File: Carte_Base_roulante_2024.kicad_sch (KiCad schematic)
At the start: 33 parts, among them J1 Screw_Terminal_01x02, J16 Screw_Terminal_01x02, J2 Screw_Terminal_01x02, J26 Conn_01x04_Male, J27 Conn_01x04_Male, J28 Conn_01x04_Male, J3 Screw_Terminal_01x02, J8 USB_B_Micro, J9 Conn_01x05, U1 STM32G484RETx, U4 R-78E5.0-1.0

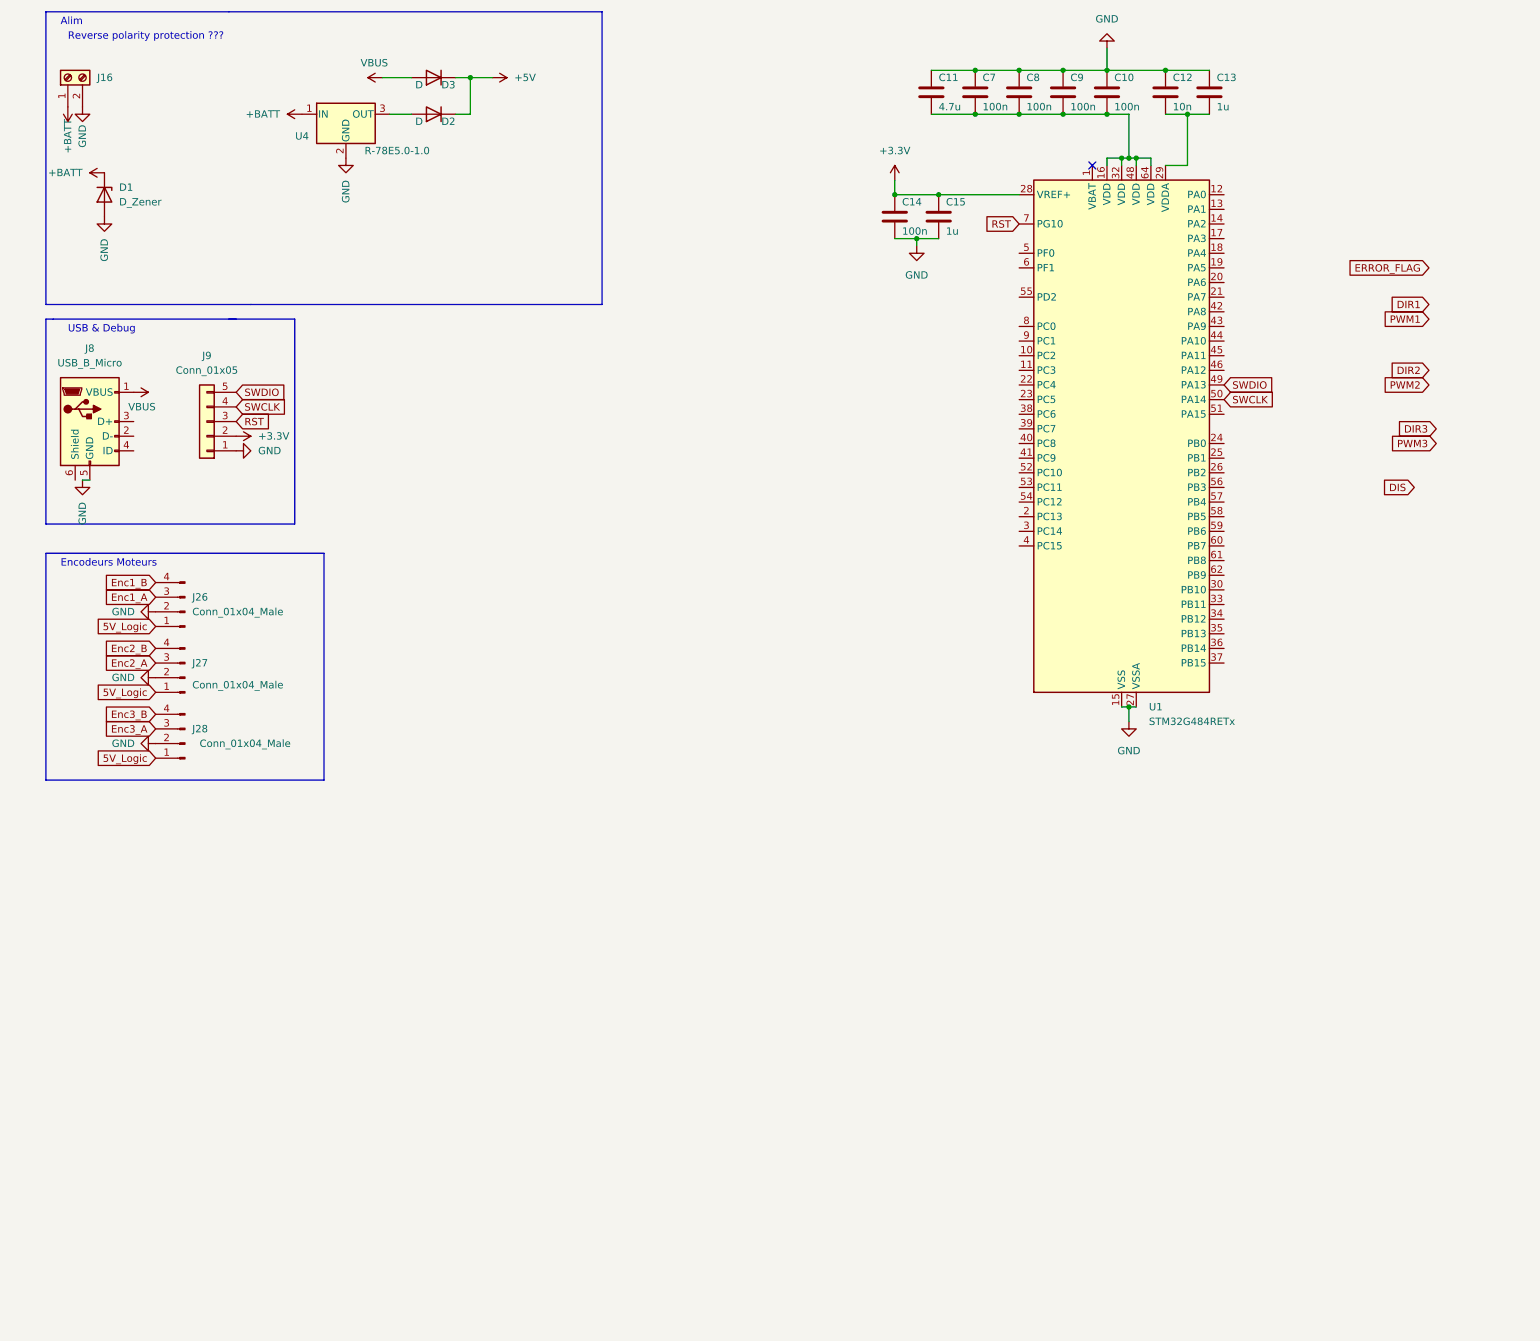
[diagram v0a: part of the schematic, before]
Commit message: IMU + SPI
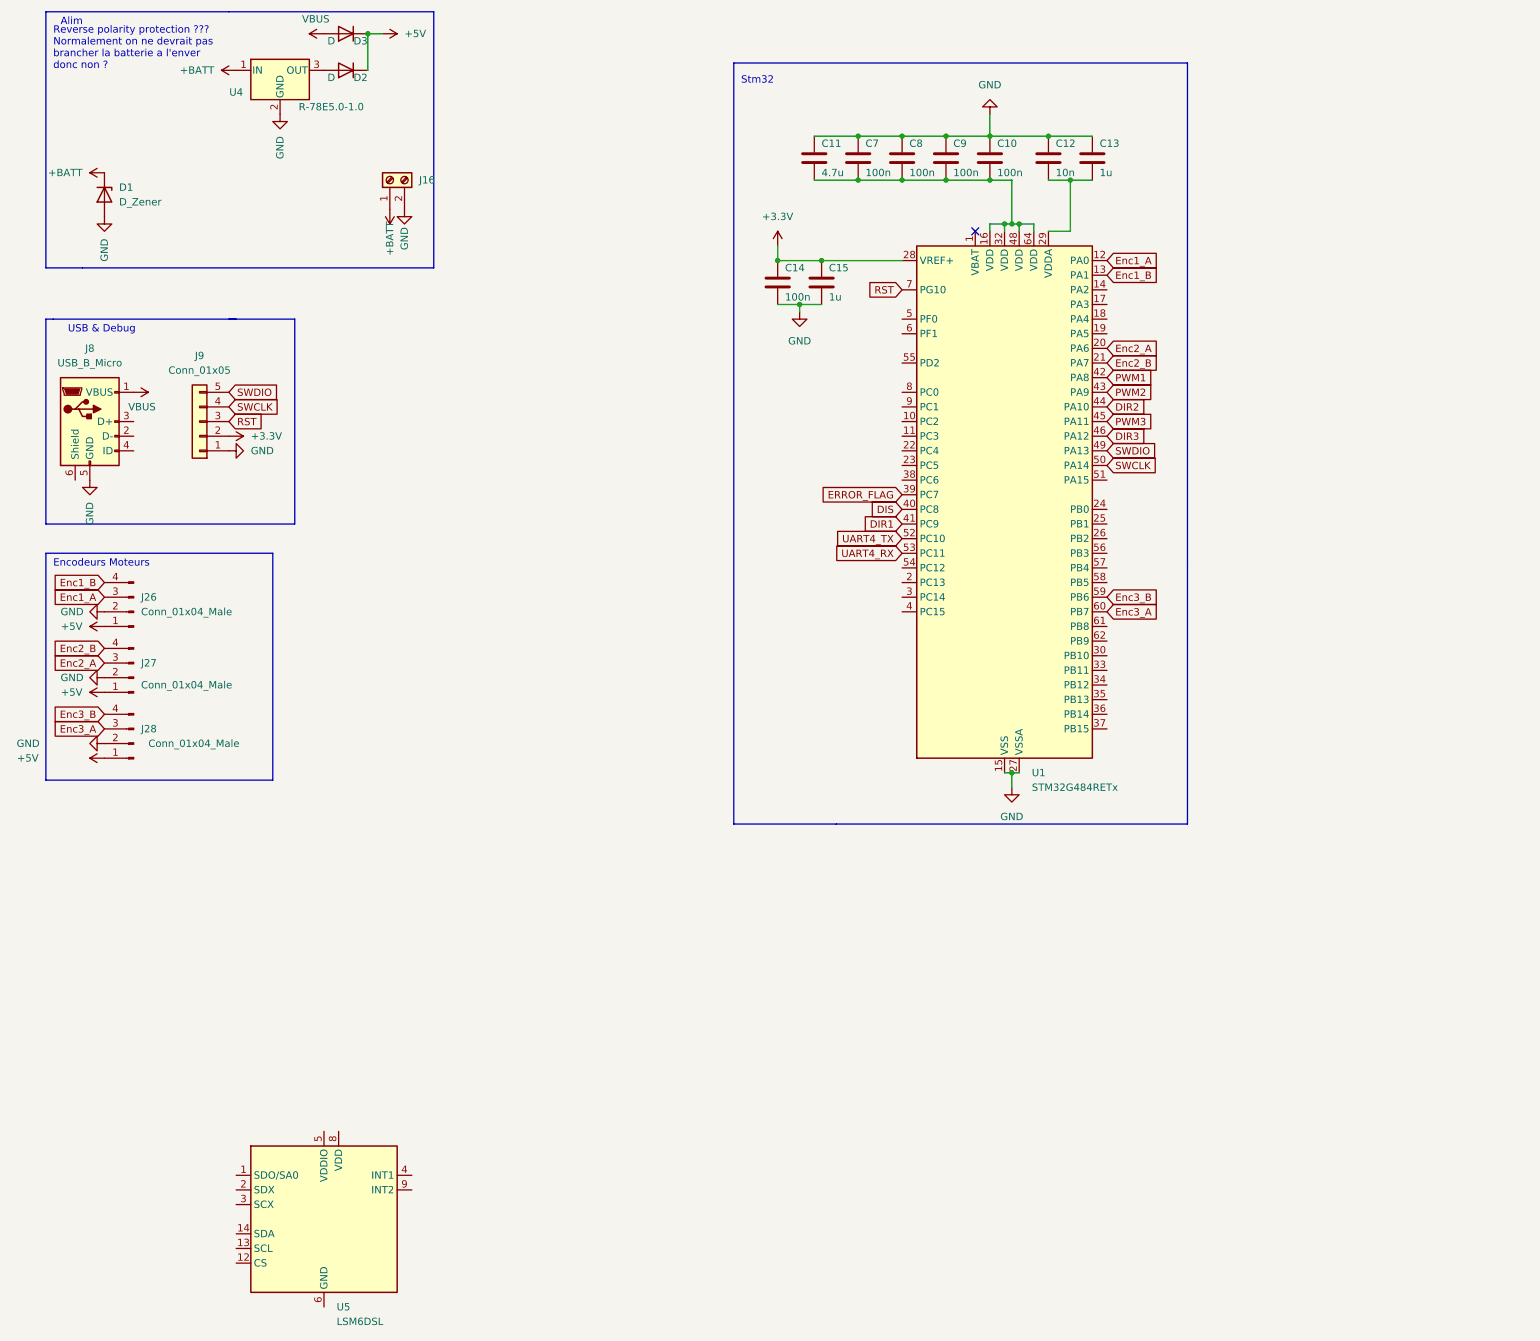
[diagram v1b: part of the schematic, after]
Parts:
- added U5: LSM6DSL, Package_LGA:LGA-14_3x2.5mm_P0.5mm_LayoutBorder3x4y, symbol Sensor_Motion:LSM6DSL
- U?: RS (none) -> https://fr.rs-online.com/web/p/drivers-de-moteur/1702333
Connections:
- net 5V_Logic is gone; now on net +5V: J26.1 (Pin_1), J27.1 (Pin_1), J28.1 (Pin_1)
- net DIR1: now also U1.41 (PC9)
- net DIR2: now also U1.44 (PA10)
- net DIR3: now also U1.46 (PA12)
- net DIS: now also U1.40 (PC8)
- net ERROR_FLAG: now also U1.39 (PC7)
- net Enc1_A: now also U1.12 (PA0)
- net Enc1_B: now also U1.13 (PA1)
- net Enc2_A: now also U1.20 (PA6)
- net Enc2_B: now also U1.21 (PA7)
- net Enc3_A: now also U1.60 (PB7)
- net Enc3_B: now also U1.59 (PB6)
- net PWM1: now also U1.42 (PA8)
- net PWM2: now also U1.43 (PA9)
- net PWM3: now also U1.45 (PA11)
- net UART4_TX: now reaches U1.52 (PC10)
- net UART4_RX: now reaches U1.53 (PC11)
- new net: U5.6 (GND), U5.7 (GND)
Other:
- note added: "Reverse polarity protection ??? Normalement on ne devrait pas brancher la batterie a l'enver donc non ?"
- note added: "Stm32"
- note removed: "Reverse polarity protection ???"
- moved on the sheet: C10, C11, C12, C13, C14, C15, C7, C8, C9, D2, D3, J16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

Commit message: usb + protection + cristal + leds + adc
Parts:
- removed J8: USB_B_Micro, symbol Connector:USB_B_Micro
- added C16, C17, C18: 100n, Capacitor_SMD:C_0805_2012Metric, symbol Device:C
- added D4: D_Zener, symbol Device:D_Zener
- added D5, D6, D7: LED, LED_SMD:LED_0603_1608Metric_Pad1.05x0.95mm_HandSolder, symbol Device:LED
- added J10: USB-C_12pin, ENAC_robotique:USB-C_HRO_C-31-M-12, symbol ENAC_robotique:USB-C_12pin
- added J8: Conn_01x03_Pin, Connector_PinHeader_2.54mm:PinHeader_1x03_P2.54mm_Vertical, symbol Connector:Conn_01x03_Pin
- added Q1: PMOS, symbol Simulation_SPICE:PMOS
- added R10, R5, R6: osef, Resistor_SMD:R_0805_2012Metric, symbol Device:R
- added R2, R3, R4: 10k, Resistor_SMD:R_0805_2012Metric, symbol Device:R
- added R7, R8: 5.1K, Resistor_SMD:R_0603_1608Metric_Pad0.98x0.95mm_HandSolder, symbol Device:R
- added R9: 40K, Resistor_SMD:R_0603_1608Metric_Pad0.98x0.95mm_HandSolder, symbol Device:R
- added SW1: SW_Push, symbol Switch:SW_Push
- added X1: ASCO, ENAC_robotique:Osc_ASCO, symbol ENAC_robotique:ASCO
- C11, C12, C13, C15: footprint (none) -> Capacitor_SMD:C_0805_2012Metric
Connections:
- net +3.3V: now also U5.5 (VDDIO), U5.8 (VDD), C16.2, C17.2, C18.1, SW1.1, X1.1 (TS), X1.4 (VDD)
- net +5V: now also R5.1
- net +BATT: now also D4.1 (K), Q1.3 (S); no longer J16.1 (Pin_1)
- net DIR1: now also U1.34 (PB12); no longer U1.41 (PC9)
- net DIR2: now also U1.33 (PB11); no longer U1.44 (PA10)
- net DIR3: now also U1.38 (PC6); no longer U1.46 (PA12)
- net DIS: now also U1.39 (PC7); no longer U1.40 (PC8)
- net ERROR_FLAG: now also U1.40 (PC8); no longer U1.39 (PC7)
- net GND: now also J16.1 (Pin_1), U5.2 (SDX), U5.3 (SCX), U5.6 (GND), U5.7 (GND), C16.1, C17.1, C18.2, D5.1 (K), D6.1 (K), D7.1 (K), J10.A1-B12 (GND), J10.B1-A12 (GND), J10.S (Shield), J8.1 (Pin_1), R2.2, R4.2, R7.2, R8.2, R9.2, X1.2 (GND); no longer J16.2 (Pin_2)
- net PWM1: now also U1.35 (PB13); no longer U1.42 (PA8)
- net PWM2: now also U1.36 (PB14); no longer U1.43 (PA9)
- net PWM3: now also U1.37 (PB15); no longer U1.45 (PA11)
- net UART4_RX: now also J8.2 (Pin_2)
- net UART4_TX: now also J8.3 (Pin_3)
- net VBUS: now also J10.A4-B9 (VBUS), J10.B4-A9 (VBUS)
- net OSCILATEUR: now reaches U1.5 (PF0)
- net OSCILATEUR: now also X1.3 (OUT)
- net IMU_INT1: now reaches U1.54 (PC12)
- net IMU_INT1: now also U5.4 (INT1)
- net SPI1_CS_IMU: now reaches U1.55 (PD2)
- net SPI1_CS_IMU: now also U5.12 (CS)
- net SPI1_SCK: now reaches U1.56 (PB3)
- net SPI1_SCK: now also U5.13 (SCL)
- net SPI1_MISO: now reaches U1.57 (PB4)
- net SPI1_MISO: now also U5.1 (SDO/SA0)
- net SPI1_MOSI: now reaches U1.58 (PB5)
- net SPI1_MOSI: now also U5.14 (SDA)
- net BOOT 0: now reaches U1.61 (PB8)
- net BOOT 0: now also R9.1, SW1.2
- new net: D5.2 (A), R5.2
- new net: D6.2 (A), R6.2
- new net: D4.2 (A), Q1.2 (G), R2.1
- new net: D7.2 (A), R10.2
- new net: J16.2 (Pin_2), Q1.1 (D), R3.1
- new net: J10.A5 (CC1), R7.1
- new net: J10.B5 (CC2), R8.1
- new net LED1: R10.1, U1.43 (PA9)
- new net LED2: R6.1, U1.44 (PA10)
- new net MEAS_VBAT: R3.2, R4.1, U1.42 (PA8)
- new net USB_DM: J10.A7 (D-1), J10.B7 (D-2), U1.45 (PA11)
- new net USB_DP: J10.A6 (D+1), J10.B6 (D+2), U1.46 (PA12)
- no-connect marks 1 -> 25
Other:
- note added: "Connectique USB UART DEBUG"
- note added: "Horloge"
- note added: "IMU"
- note added: "LEDS"
- note added: "valeurs des R_leds marqué "osef" car pn peux voir ça après ( il y en a 3 )"
- note removed: "Reverse polarity protection ??? Normalement on ne devrait pas brancher la batterie a l'enver donc non ?"
- note removed: "USB & Debug"
- moved on the sheet: C1, C10, C11, C12, C13, C14, C15, C2, C3, C4, C5, C6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
